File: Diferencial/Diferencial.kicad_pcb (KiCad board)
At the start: 2 copper layers, 99.1 x 140.1 mm, 105 parts, among them J1 Pedal Sensor 1, J2 Pedal Sensor 2, J3 Brake Sensor 1, J4 Brake Sensor 2, J5 Out_Brake_Light, J6 Buzzer_out, J7 DB9_Female, J8 DB9_Female, K1 RELAY_19.1x15.5mm, Q1 MMBT3904, Q2 MMBT3904, U1 LM358, U2 UFRGS_PILL, U3 LM358, U4 MCP2558FD-xSN, U5 LM317_TO39

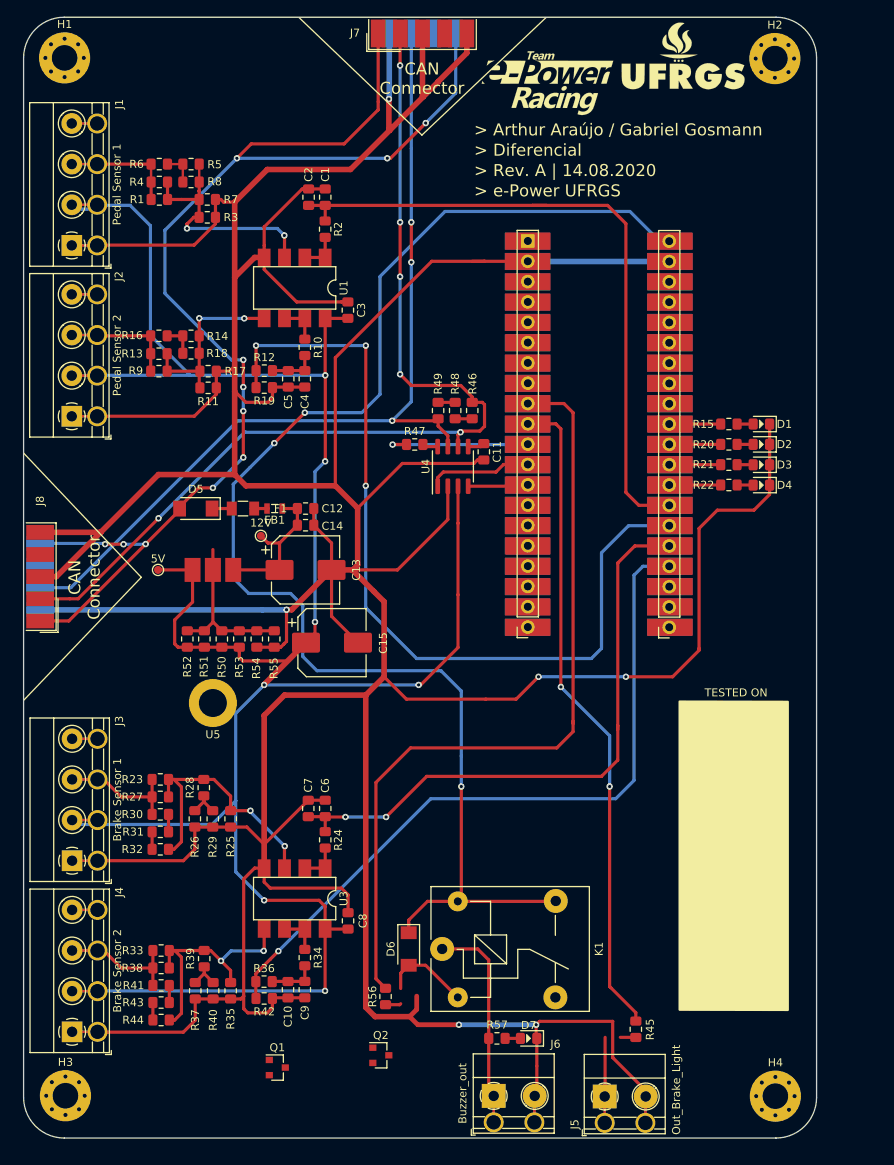
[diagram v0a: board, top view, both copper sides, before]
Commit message: Diferencial Layout Update
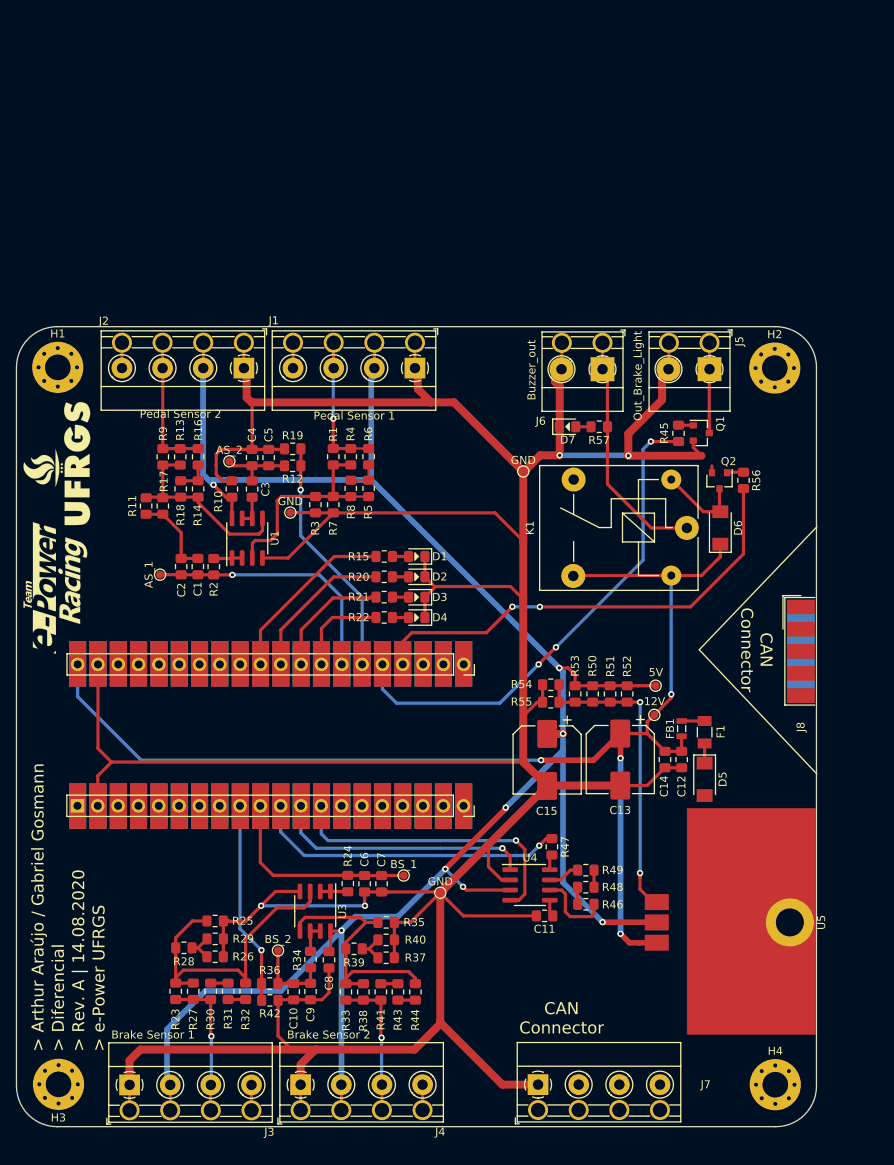
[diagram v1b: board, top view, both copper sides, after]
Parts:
- added TP3: AS_1, e-Power:TestPoint_Pad_D1.0mm, F.Cu at (83.0, 99.3)
- added TP4: AS_2, e-Power:TestPoint_Pad_D1.0mm, F.Cu at (91.7, 85.1)
- added TP5: GND, e-Power:TestPoint_Pad_D1.0mm, F.Cu at (118.0, 139.0)
- added TP6: BS_1, e-Power:TestPoint_Pad_D1.0mm, F.Cu at (113.4, 136.9)
- added TP7: BS_2, e-Power:TestPoint_Pad_D1.0mm, F.Cu at (97.7, 146.2)
- added TP8: GND, e-Power:TestPoint_Pad_D1.0mm, F.Cu at (99.3, 91.5)
- added TP9: GND, e-Power:TestPoint_Pad_D1.0mm, F.Cu at (128.4, 86.3)
- J7: value DB9_Female -> Screw_Terminal_01x04; footprint e-Power:DSUB-9_Female_EdgeMount_P2.77mm -> e-Power:TerminalBlock_Phoenix_MKDS-1,5-4-5.08_1x04_P5.08mm_Horizontal
- U1, U3: footprint e-Power:DIP-8_SMD -> Package_SO:SOIC-8_3.9x4.9mm_P1.27mm
- U5: value LM317_TO39 -> LM317_3PinPackage
- moved J7 132.2 mm to (130.2, 163.0), turned to 0 degrees
- moved J8 95.6 mm to (163.1, 108.8), turned to 90 degrees
- moved Q1 95.4 mm to (150.7, 81.5)
- moved G1 93.4 mm to (70.1, 85.3), turned to 90 degrees
- moved J5 91.9 mm to (151.7, 73.6), turned to 180 degrees
- moved J6 91.8 mm to (138.3, 73.6), turned to 180 degrees
- moved G2 88.1 mm to (69.9, 100.9), turned to 90 degrees
- moved Q2 83.4 mm to (152.9, 87.5), turned to 270 degrees
- moved R56 78.5 mm to (155.9, 87.5), turned to 90 degrees
- moved R57 77.5 mm to (137.9, 80.8), turned to 0 degrees
- moved D7 76.6 mm to (133.9, 80.8), turned to 0 degrees
- moved R45 74.7 mm to (147.8, 81.6), turned to 270 degrees
- moved D5 72.0 mm to (151.1, 124.8), turned to 270 degrees
- moved U5 67.3 mm to (145.1, 140.2), turned to 270 degrees
- moved D6 65.5 mm to (153.0, 93.4), turned to 90 degrees
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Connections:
- J7 pad 1: /Input_Power -> GND
- J7 pad 3: GND -> /CAN_H
- J7 pad 4: (no net) -> /Input_Power
- U2 pad 10: /Brake_Light -> /Brake_Sensor_1
- U2 pad 24: /Brake_Sensor_2 -> /Ready_to_Drive
- U2 pad 25: /Brake_Sensor_1 -> /Brake_Light
- U2 pad 9: /Ready_to_Drive -> /Brake_Sensor_2
- U5 pad 1: +12V -> Net-(R50-Pad2)
- U5 pad 2: Net-(R50-Pad2) -> +5V
- U5 pad 3: +5V -> +12V
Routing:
- net GND: track 792.8 -> 596.0 mm, vias 6 -> 4
- net /Input_Power: track 161.3 -> 0.40 mm, vias 11 -> 0
- net /CAN_L: track 124.3 -> 9.60 mm, vias 6 -> 0
- net /CAN_H: track 111.9 -> 4.35 mm, vias 3 -> 0
- net /ACC_Sensor_2: track 106.2 -> 30.1 mm, vias 3 -> 1
- net /Brake_Sensor_2: track 90.9 -> 25.4 mm
- net /ACC_Sensor_1: track 84.0 -> 32.3 mm, vias 0 -> 1
- net /Brake_Sensor_1: track 76.0 -> 25.7 mm, vias 2 -> 0
- net /Ready_to_Drive: track 99.8 -> 63.1 mm, vias 0 -> 2
- net +12V: track 195.3 -> 159.9 mm, vias 3 -> 4
- net /RX: track 7.53 -> 37.5 mm, vias 0 -> 1
- net /S: track 18.7 -> 39.3 mm
- net /Brake_Light: track 82.3 -> 62.5 mm, vias 2 -> 3
- net /TX: track 13.0 -> 32.4 mm, vias 0 -> 1
- net Net-(R50-Pad2): track 20.8 -> 38.5 mm, vias 0 -> 2
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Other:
- board size 99.1 x 140.1 mm -> 100 x 100 mm
